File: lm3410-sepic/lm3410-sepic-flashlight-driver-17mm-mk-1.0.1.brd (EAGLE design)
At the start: 17.4 x 17.4 mm, 16 parts, among them Q1 PSMN2R4-30MLD, U1 ATTINY13a, U2 PAM2803

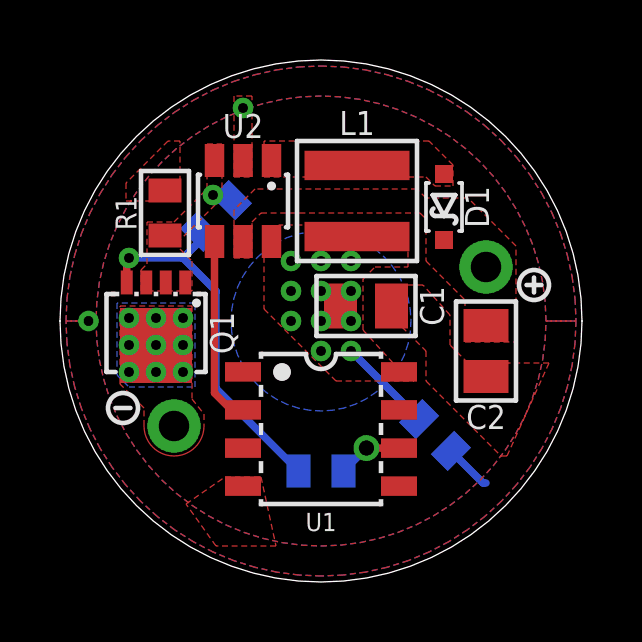
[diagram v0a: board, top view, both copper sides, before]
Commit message: bunch of new board word
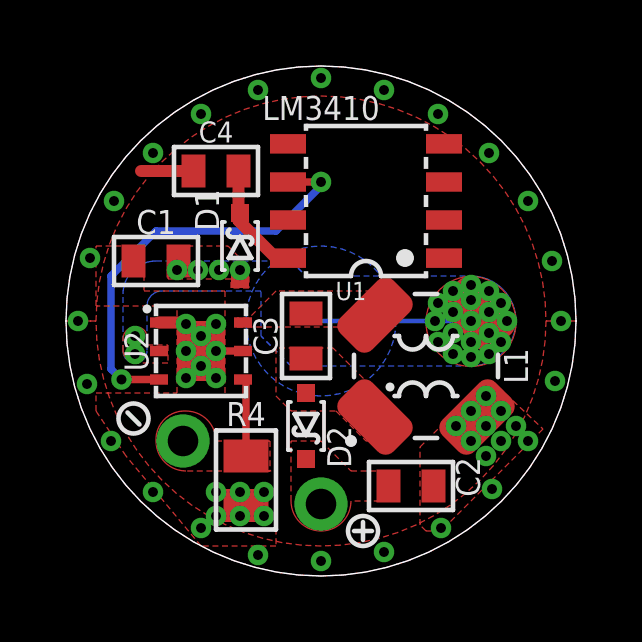
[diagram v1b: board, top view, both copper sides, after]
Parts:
- removed A, K: M01PTH-1MM-CIR-NS, a_parts:1X01-1MM-CIR-NS
- removed Q1: PSMN2R4-30MLD, a_parts:LFPAK33
- removed R1: 0R1, a_parts:R0603-TIGHTER
- removed R2: 150K, a_parts:R0603-TIGHTER
- removed R3: 33K, a_parts:R0603-TIGHTER
- added C3: 2u2, a_parts:C0603-TIGHTER
- added C4: 1u, a_parts:C0603-TIGHTER
- added D2: BAT60A, a_parts:SOD323-SCHOTTKY
- added LED+, LED-: M01PTH-1MM-CIR-NS, a_parts:1X01-1MM-CIR-NS
- C1: value 10uF -> 10u; device a_parts:C0805-TIGHTER -> a_parts:C0603-TIGHTER
- C2: value 22uF -> 10u; device a_parts:C0805-TIGHTER -> a_parts:C0603-TIGHTER
- D1: value BAT60 -> BAT60A
- L1: value 2.2uF -> 1uH; device a_parts:XFL4020 -> a_parts:LPD5030
- R4: value 33R -> X; device a_parts:R0603-TIGHTER -> a_parts:R0805-TIGHTER
- U1: value ATTINY13a -> Tiny25
- U2: value PAM2803 -> LM3410XSDNGG; device a_parts:SOT23-6 -> a_parts:DFN300X300X80-7N
- moved U1 7.75 mm to (10.0, 12.5), turned to 90 degrees
- moved C1 7.16 mm to (3.00, 10.5), turned to 180 degrees
- moved D1 6.92 mm to (5.80, 11.0), turned to 90 degrees
- moved + 6.00 mm to (13.5, 8.50), turned to 180 degrees
- moved L1 5.96 mm to (12.0, 7.00), turned to 90 degrees
- moved U2 5.19 mm to (4.50, 7.50), turned to 0 degrees
- moved C2 5.15 mm to (11.5, 3.00), turned to 0 degrees
- moved R4 2.52 mm to (6.00, 3.20), flipped to the top, turned to 90 degrees
- moved - 0.35 mm to (0.40, 8.50), flipped to the bottom
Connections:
- removed net !SHDN: U1.2, U2.4
- removed net GATE: Q1.4, R3.2, R4.2
- removed net LED-: K.1, Q1.PAD
- new net N$1: C3.2, D2.A, L1.1
- new net VCC: C4.1, D1.C, U1.8
- net FB: now also LED-.1, R4.2, U2.4; no longer Q1.1, Q1.2, Q1.3, R1.2, R3.1, U2.3
- net GND: now also C4.2, L1.2, R4.1, U2.1, U2.5, U2.PAD; no longer R1.1, R2.1, U2.2
- net LED+: now also D2.C, LED+.1; no longer A.1, D1.C, U2.5
- net PWM: now also U2.3; no longer R4.1
- net SW: now also C3.1, L1.4, U2.6; no longer D1.A, L1.P$1, U2.1
- net VBAT: now also D1.A, L1.3, U2.2; no longer L1.P$2, R2.2, U1.8, U2.6
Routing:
- net GATE: track 12.4 -> 0.00 mm, vias 1 -> 0
- net PWM: track 2.17 -> 14.3 mm, vias 1 -> 2
- net !SHDN: track 6.23 -> 0.00 mm
- net VCC: track 0.00 -> 4.07 mm
- net GND: track 1.61 -> 3.57 mm, vias 1 -> 46
- net FB: track 0.80 -> 2.65 mm, vias 1 -> 0
- net VBAT: track 3.21 -> 5.00 mm, vias 10 -> 24
- added copper zone on layer 1, net N$1
- removed copper zone on layer 1, net LED-
- removed copper zone on layer 16, net LED-
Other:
- board size 17.4 x 17.4 mm -> 17 x 17 mm
- board text added: "0.2 --- R4"
- board text added: "Iout="
- board text added: "LM3410"
- board text added: "LM3410 SEPIC LED Drv"
- board text added: "Vin 2.5-4.5V"
- board text removed: "17mm"
- board text removed: "Boost Driver"
- board text removed: "PAM2803"
- board text removed: "~"
